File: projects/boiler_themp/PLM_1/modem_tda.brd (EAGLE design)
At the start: 50 x 50 mm, 17 parts, among them IC1 TDA5051, X1 8MHz

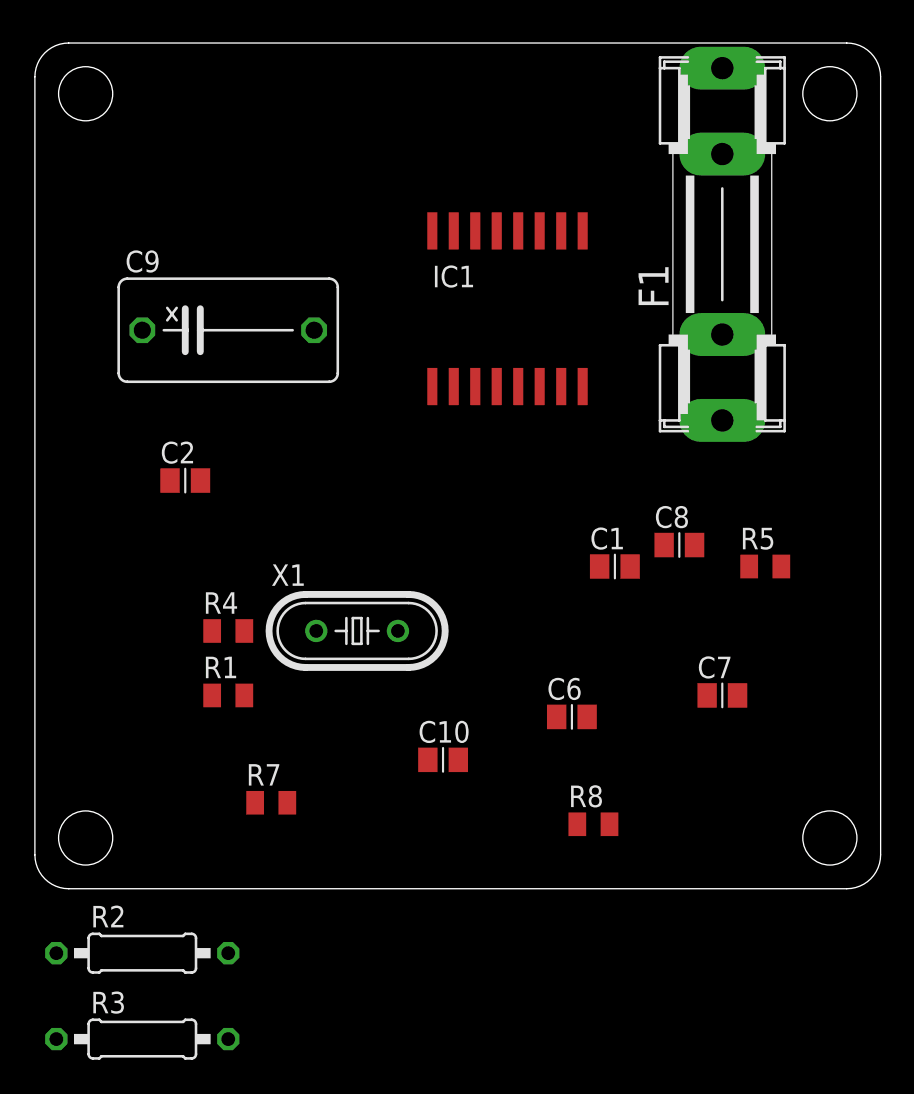
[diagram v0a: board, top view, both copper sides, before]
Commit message: PLM Version 1.0 Finished and sent to PCB house
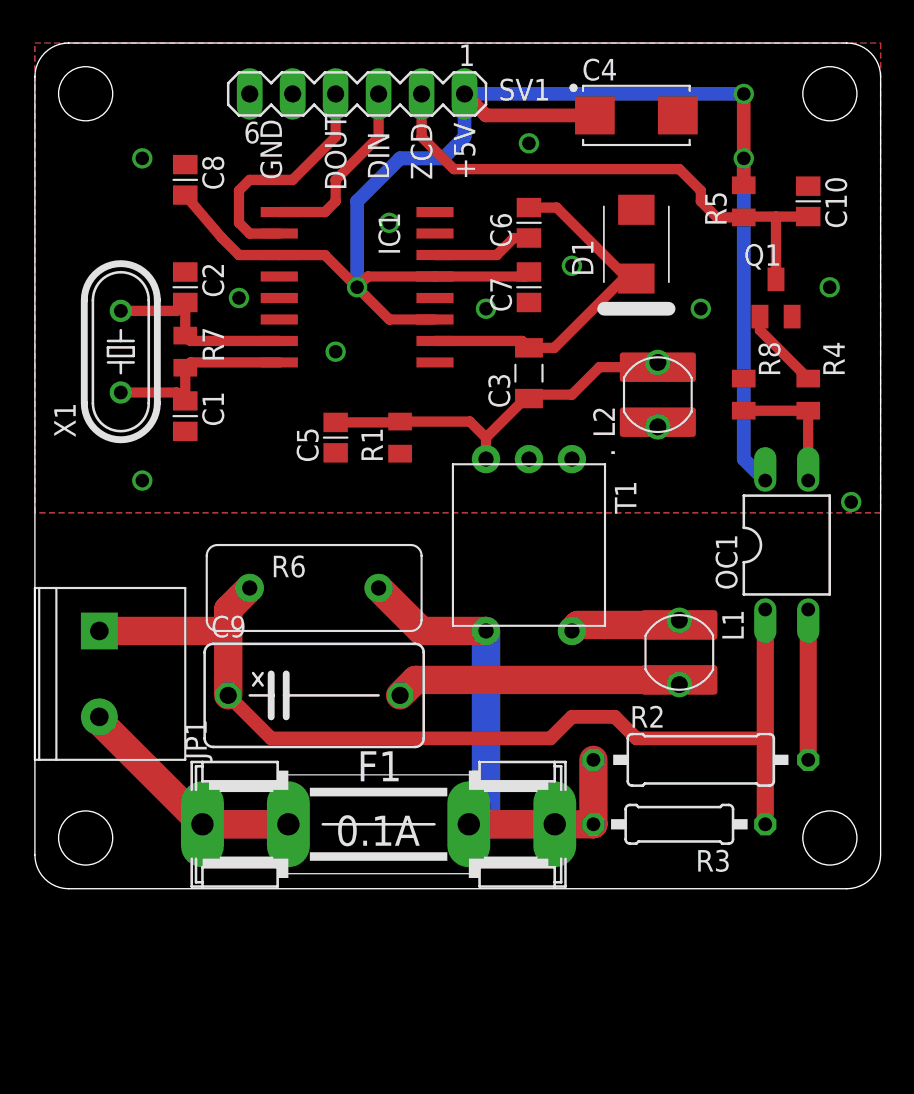
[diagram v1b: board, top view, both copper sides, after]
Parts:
- added C3: 10 uF 16V, ipc-7351-capacitor:CAPC3215X168N
- added C4: 100 uF, ipc-7351-capacitor:CAPMP6032X150N
- added C5: 0.1uF, ipc-7351-capacitor:CAPC2012X145AN
- added D1: SMBJ7.0A, diode:SMBJ
- added JP1: (no value), jlab:BLUE_TERM
- added L1: 47 uH, jlab_varistors:CD43
- added L2: 22 uH, jlab_varistors:CD43
- added OC1: PC814, optocoupler:DIL04
- added Q1: 2N3904SOT23, transistor-npn:SOT23-BEC
- added R6: 10D391K, jlab_varistors:MOV-10D
- added SV1: (no value), con-lstb:MA06-1
- added T1: MU-78250, jlab:6-PIN-DIL
- R2: device rcl:0207/10 -> rcl:0309/12
- moved F1 39.9 mm to (20.3, 3.81), turned to 0 degrees
- moved C10 39.5 mm to (45.7, 40.6), turned to 270 degrees
- moved R4 37.0 mm to (45.7, 29.2), turned to 90 degrees
- moved C8 36.3 mm to (8.89, 41.9), turned to 270 degrees
- moved R2 34.9 mm to (39.4, 7.62)
- moved R3 34.2 mm to (38.1, 3.81), turned to 180 degrees
- moved C6 29.3 mm to (29.2, 39.4), turned to 90 degrees
- moved R7 27.1 mm to (8.89, 31.8), turned to 90 degrees
- moved R8 26.9 mm to (41.9, 29.2), turned to 270 degrees
- moved C1 26.9 mm to (8.89, 27.9), turned to 270 degrees
- moved C7 26.7 mm to (29.2, 35.6), turned to 90 degrees
- moved C9 22.2 mm to (16.5, 11.4)
- moved R5 21.6 mm to (41.9, 40.6), turned to 90 degrees
- moved X1 21.6 mm to (5.08, 31.8), turned to 90 degrees
- moved R1 18.3 mm to (21.6, 26.7), turned to 90 degrees
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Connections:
- new net +5V: C4.+, C7.2, C8.2, IC1.11, IC1.13, IC1.3, OC1.4, R5.2, SV1.1
- new net GND: C1.2, C10.1, C2.2, C4.-, C5.1, C7.1, C8.1, D1.A, IC1.12, IC1.5, IC1.9, L2.1, Q1.E, R1.1, R8.1, SV1.5, SV1.6, T1.1
- new net N$1: F1.1A, F1.1B, JP1.2
- new net N$10: C10.2, Q1.C, R5.1, SV1.2
- new net N$11: C6.1, IC1.14
- new net N$12: C2.1, IC1.7, R7.2, X1.2
- new net N$13: C1.1, IC1.8, R7.1, X1.1
- new net N$14: IC1.1, SV1.3
- new net N$15: IC1.2, SV1.4
- new net N$16: Q1.B, R4.2
- new net N$2: F1.2A, F1.2B, R2.1, R3.2, R6.2, T1.4
- new net N$3: C9.1, JP1.1, OC1.1, R3.1, R6.1
- new net N$4: OC1.2, R2.2
- new net N$5: C9.2, L1.2
- new net N$6: L1.1, T1.6
- new net N$7: OC1.3, R4.1, R8.2
- new net N$8: C3.1, C5.2, L2.2, R1.2, T1.3
- new net N$9: C3.2, C6.2, D1.C, IC1.10
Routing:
- net +5V: track 0.00 -> 93.7 mm, vias 0 -> 3
- net N$3: track 0.00 -> 61.1 mm
- net N$2: track 0.00 -> 35.9 mm
- net N$10: track 0.00 -> 31.5 mm
- net N$8: track 0.00 -> 22.5 mm, vias 0 -> 1
- net N$9: track 0.00 -> 21.9 mm
- net N$1: track 0.00 -> 19.3 mm
- net N$5: track 0.00 -> 16.9 mm, vias 0 -> 1
- net N$15: track 0.00 -> 14.1 mm
- net N$13: track 0.00 -> 11.7 mm
- net N$12: track 0.00 -> 11.7 mm
- net N$14: track 0.00 -> 11.0 mm
- net N$4: track 0.00 -> 8.89 mm
- net N$7: track 0.00 -> 7.94 mm
- net N$6: track 0.00 -> 6.50 mm, vias 0 -> 1
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- added copper zone on layer 1, net GND
- added copper zone on layer 16, net GND
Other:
- board text added: "+5V"
- board text added: "DIN"
- board text added: "DOUT"
- board text added: "GND"
- board text added: "Igor L."
- board text added: "March 2013"
- board text added: "PLM ver.1.0"
- board text added: "ZCD"
- board text added: "jungoigorl@gmail.com"
